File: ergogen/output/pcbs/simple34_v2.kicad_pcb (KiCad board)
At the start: 2 copper layers, 116.6 x 89.6 mm, 41 parts

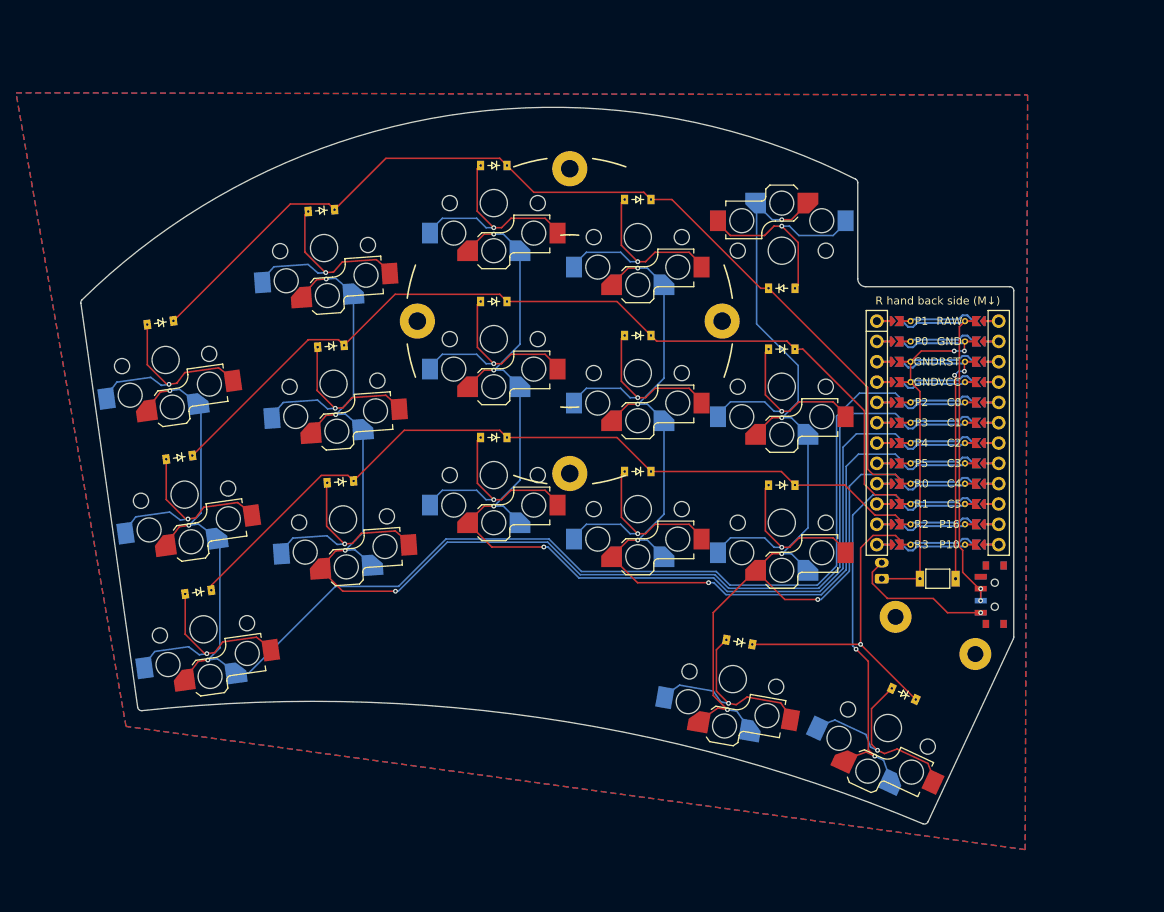
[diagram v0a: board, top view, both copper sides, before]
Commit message: LARGE UPDATE
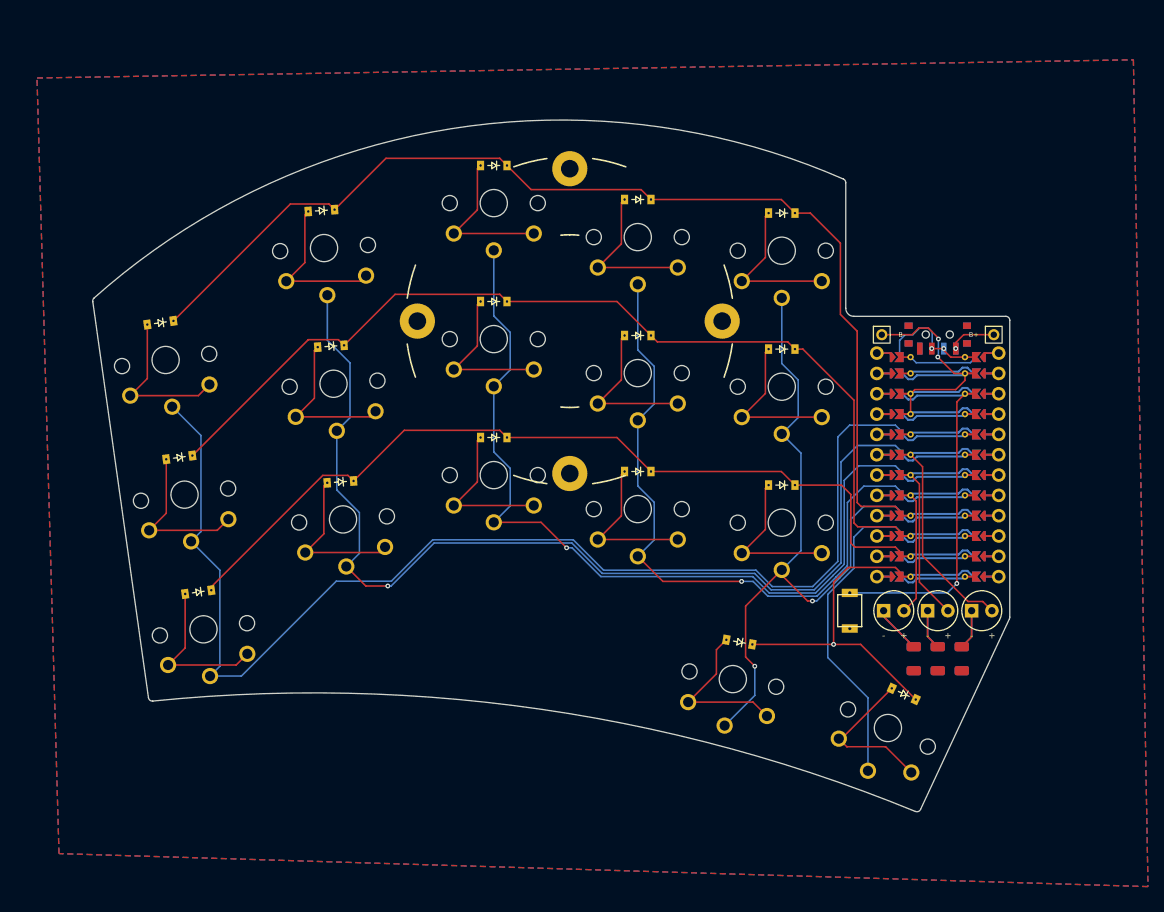
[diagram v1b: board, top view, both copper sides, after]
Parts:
- removed H1, H2: , ceoloide:mounting_hole_plated
- removed JST1: , ceoloide:battery_connector_jst_ph_2
- added BAT1: , terence:battery_socket_tht, F.Cu at (139.4, 63.3)
- added LED1: , terence:led_5mm_tht, F.Cu at (144.9, 97.8)
- added LED2: , terence:led_5mm_tht, F.Cu at (139.4, 97.8)
- added LED3: , terence:led_5mm_tht, F.Cu at (133.9, 97.8)
- added R1: , terence:resistor_1206, F.Cu at (142.4, 103.8)
- added R2: , terence:resistor_1206, F.Cu at (139.4, 103.8)
- added R3: , terence:resistor_1206, F.Cu at (136.4, 103.8)
- moved PWR1 33.3 mm to (139.4, 63.3), turned to 90 degrees
- moved SW1 11.7 mm to (128.4, 97.8), turned to 90 degrees
- moved D15 9.40 mm to (119.9, 48.1), turned to 180 degrees
- moved MCU1 4.00 mm to (139.4, 78.3)
- turned S15 to 180 degrees
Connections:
- MCU1 pad 117: P5 -> led_3
- MCU1 pad 118: P4 -> led_2
- MCU1 pad 119: P3 -> led_1
- S1 pad 1: C0 -> pinky_bottom
- S1 pad 2: pinky_bottom -> C0
- S10 pad 1: C3 -> index_bottom
- S10 pad 2: index_bottom -> C3
- S11 pad 1: C3 -> index_home
- S11 pad 2: index_home -> C3
- S12 pad 1: C3 -> index_top
- S12 pad 2: index_top -> C3
- S13 pad 1: C4 -> inner_bottom
- S13 pad 2: inner_bottom -> C4
- S14 pad 1: C4 -> inner_home
- S14 pad 2: inner_home -> C4
- S15 pad 1: C4 -> inner_top
- S15 pad 2: inner_top -> C4
- S16 pad 1: C4 -> first_only
- S16 pad 2: first_only -> C4
- S17 pad 1: C5 -> second_only
- S17 pad 2: second_only -> C5
- S2 pad 1: C0 -> pinky_home
- S2 pad 2: pinky_home -> C0
- S3 pad 1: C0 -> pinky_top
- S3 pad 2: pinky_top -> C0
- S4 pad 1: C1 -> ring_bottom
- S4 pad 2: ring_bottom -> C1
- S5 pad 1: C1 -> ring_home
- S5 pad 2: ring_home -> C1
- S6 pad 1: C1 -> ring_top
- S6 pad 2: ring_top -> C1
- S7 pad 1: C2 -> middle_bottom
- S7 pad 2: middle_bottom -> C2
- S8 pad 1: C2 -> middle_home
- S8 pad 2: middle_home -> C2
- S9 pad 1: C2 -> middle_top
- S9 pad 2: middle_top -> C2
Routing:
- net C4: track 142.5 -> 96.8 mm, vias 5 -> 2
- net led_1: track 0.00 -> 34.6 mm
- net RAW: track 47.8 -> 15.6 mm
- net led_2: track 0.00 -> 28.7 mm
- net C3: track 120.9 -> 93.2 mm, vias 4 -> 1
- net C2: track 142.7 -> 115.2 mm, vias 4 -> 1
- net C1: track 165.4 -> 138.0 mm, vias 4 -> 1
- net led_3: track 0.00 -> 25.2 mm
- net C0: track 180.7 -> 161.5 mm, vias 3 -> 0
- net GND: track 70.4 -> 55.0 mm
- net R0: track 132.8 -> 146.2 mm
- net BAT_P: track 18.1 -> 5.91 mm
- net r3: track 0.00 -> 12.1 mm
- net r2: track 0.00 -> 10.1 mm
- net r1: track 0.00 -> 10.0 mm
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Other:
- board size 116.6 x 89.6 mm -> 114.6 x 86.5 mm

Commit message: lil change
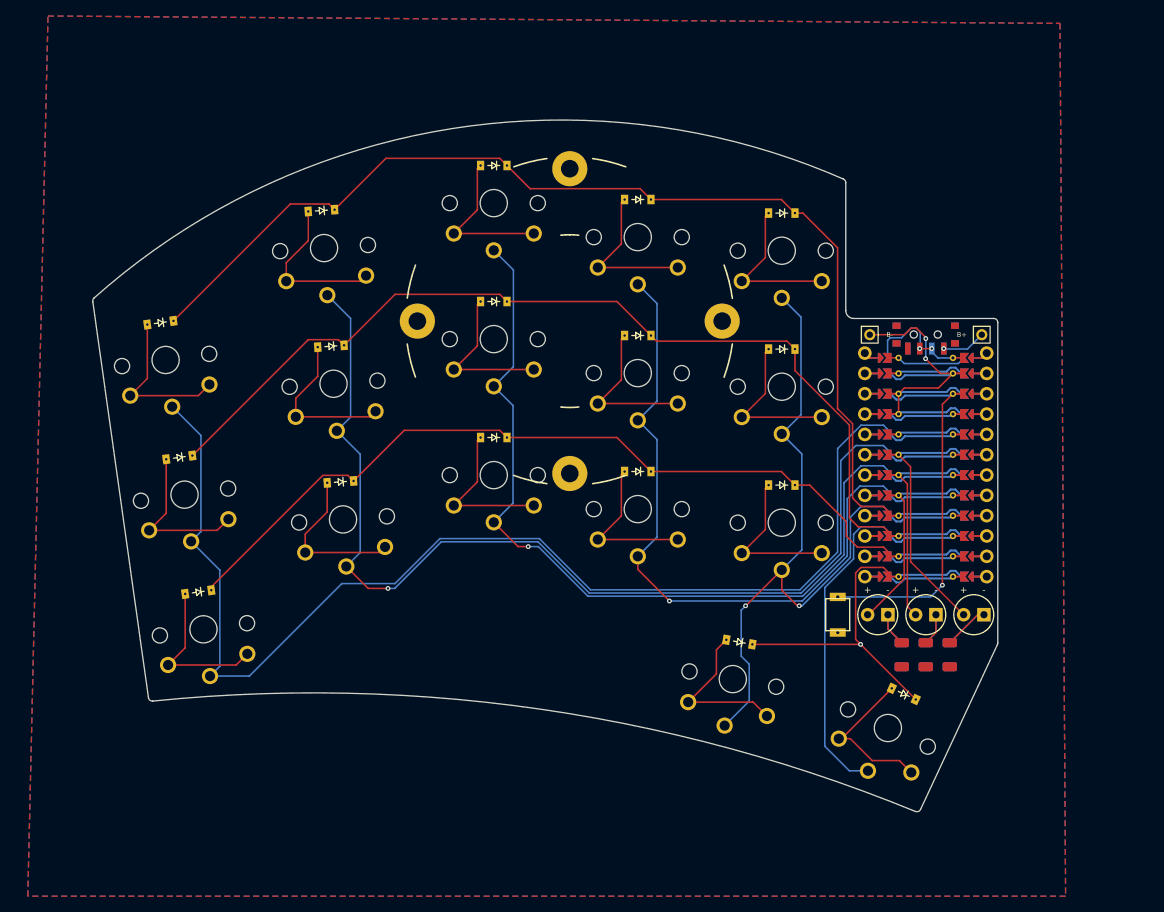
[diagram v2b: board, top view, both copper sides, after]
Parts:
- moved LED3 2.06 mm to (131.9, 98.3), turned to 180 degrees
- moved LED2 1.58 mm to (137.9, 98.3), turned to 180 degrees
- moved R1 1.58 mm to (140.9, 103.3)
- moved R2 1.58 mm to (137.9, 103.3)
- moved R3 1.58 mm to (134.9, 103.3)
- moved SW1 1.58 mm to (126.9, 98.3)
- moved BAT1 1.50 mm to (137.9, 63.3)
- moved MCU1 1.50 mm to (137.9, 78.3)
- moved PWR1 1.50 mm to (137.9, 63.3)
- moved LED1 1.12 mm to (143.9, 98.3), turned to 180 degrees
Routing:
- net R2: track 115.4 -> 111.4 mm
- net r3: track 12.1 -> 8.43 mm
- net R3: track 50.7 -> 47.4 mm
- net C0: track 161.5 -> 158.9 mm
- net R1: track 129.0 -> 126.9 mm
- net R0: track 146.2 -> 144.2 mm
- net r2: track 10.1 -> 8.05 mm
- net led_3: track 25.2 -> 27.0 mm
- net C2: track 115.2 -> 113.8 mm
- net r1: track 10.0 -> 11.4 mm
- net led_1: track 34.6 -> 33.2 mm
- net C1: track 138.0 -> 136.7 mm
- net led_2: track 28.7 -> 28.2 mm
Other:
- board size 114.6 x 86.5 mm -> 113.1 x 86.5 mm
